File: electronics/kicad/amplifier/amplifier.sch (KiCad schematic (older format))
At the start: 14 parts, among them U1 BFP620

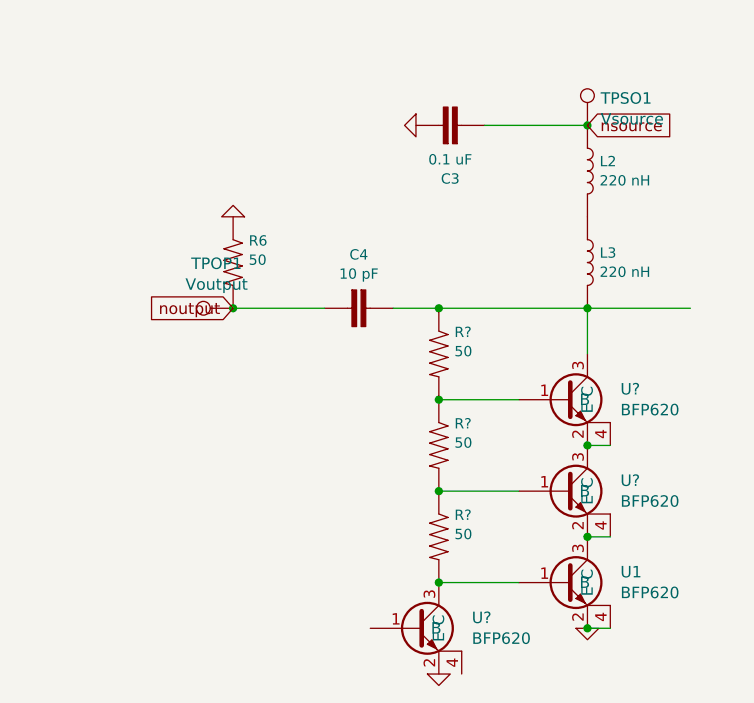
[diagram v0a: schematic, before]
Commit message: VCO
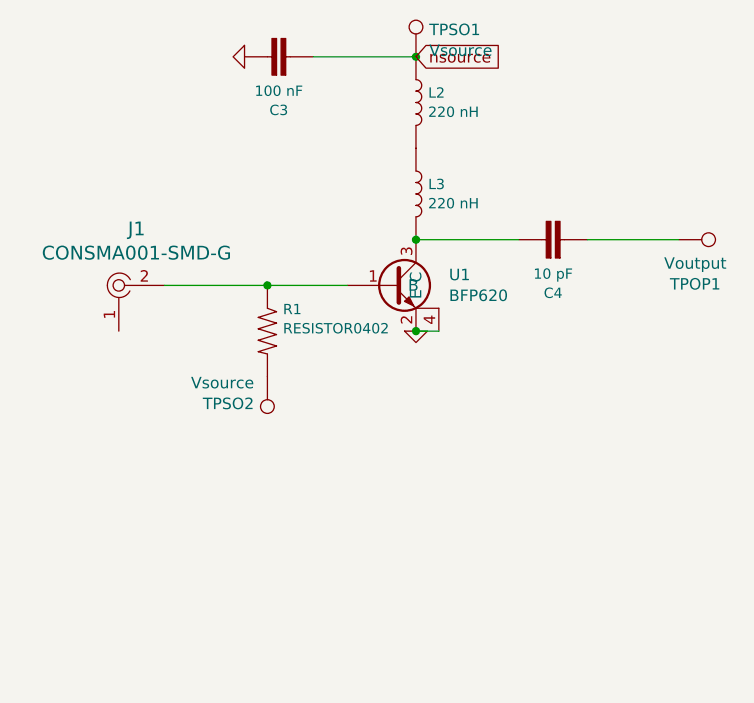
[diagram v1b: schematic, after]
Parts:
- removed R6, R? (x3): 50, Resistor_SMD:R_0402_1005Metric, symbol SparkFun-Resistors:RESISTOR0402
- removed U1, U? (x2): BFP620, Package_TO_SOT_SMD:SOT-343_SC-70-4, symbol 0xDBFB7:BFP620
- added J1: CONSMA001-SMD-G, digikey-footprints:RF_SMA_Receptical_Vertical_CONSMA001-SMD-G, symbol dk_Coaxial-Connectors-RF:CONSMA001-SMD-G
- added R1: RESISTOR0402, 0402, symbol SparkFun-Resistors:RESISTOR0402
- added TPSO2: Vsource, TestPoint:TestPoint_Pad_2.0x2.0mm, symbol Connector:Test_Point
- C3: value 0.1 uF -> 100 nF
- gave numbers to parts that had none: 1
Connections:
- net labels removed: noutput
- wire segments 12 -> 6
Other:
- moved on the sheet: C3, C4, L2, L3, TPOP1, TPSO1, U1
